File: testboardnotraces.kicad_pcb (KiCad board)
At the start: 2 copper layers, 88 x 96 mm, 75 parts, among them J1 Conn_02x05_Odd_Even, J2 Conn_01x06, J3 Thruster_Connection, Q1 SCT2450KEC, SW1 PTS645SM43SMTR92_LFS, U1 PIC18F47K40, U10 INA233, U11 INA233, U12 TPS2557, U13 EMCO-Q50-5, U14 TPS2557, U15 EMCO-Q50-5, U16 MAX6675, U2 MAX6816, U3 WPMDM171050601, U4 WPMDM171050601, U5 MAX5483, U6 EMCO-Q10-5, U7 INA233, U8 INA233, U9 INA233

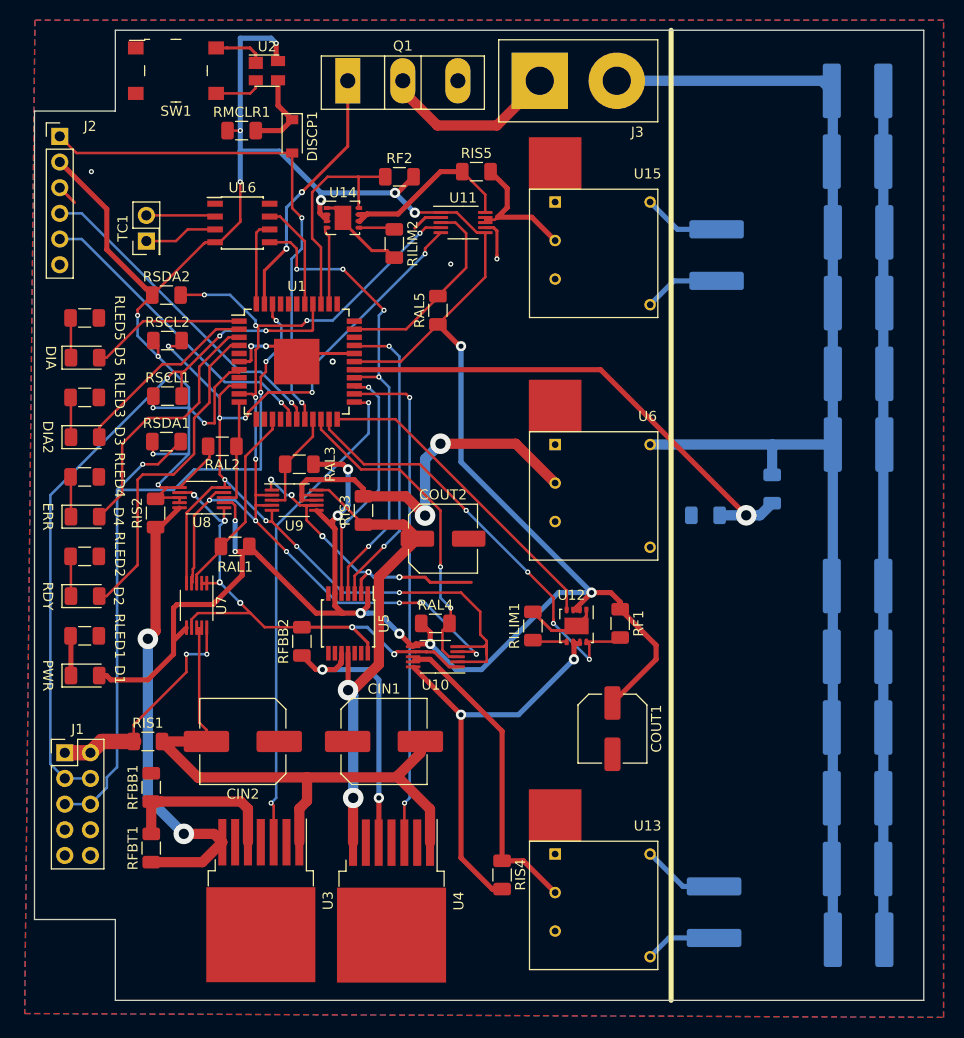
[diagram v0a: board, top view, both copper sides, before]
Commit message: Board design 1
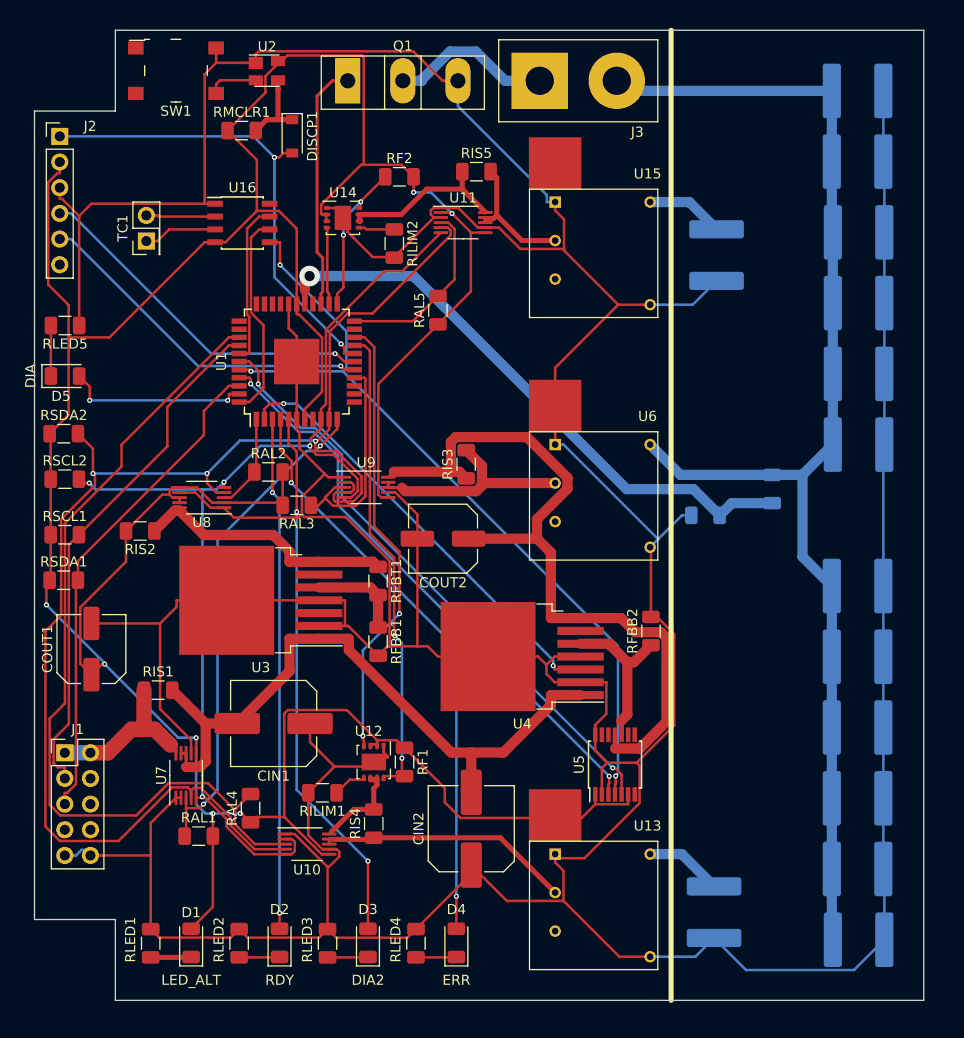
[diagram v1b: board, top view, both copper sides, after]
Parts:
- D1: value PWR -> LED_ALT
- moved RLED3 59.1 mm to (127.0, 139.3), turned to 270 degrees
- moved D3 57.3 mm to (131.0, 139.3), turned to 90 degrees
- moved RLED4 56.6 mm to (135.8, 139.3), turned to 270 degrees
- moved D4 55.9 mm to (139.8, 139.3), turned to 90 degrees
- moved COUT1 52.2 mm to (103.6, 110.2), turned to 90 degrees
- moved RLED2 41.2 mm to (118.2, 139.3), turned to 270 degrees
- moved D2 39.3 mm to (122.2, 139.3), turned to 90 degrees
- moved RFBT1 34.7 mm to (132.0, 103.5), turned to 270 degrees
- moved RFBB2 34.6 mm to (159.0, 108.5)
- moved RLED1 31.1 mm to (109.5, 139.3), turned to 270 degrees
- moved U5 29.9 mm to (155.4, 121.7), turned to 90 degrees
- moved U3 29.7 mm to (120.4, 105.4), turned to 180 degrees
- moved RAL1 28.9 mm to (114.2, 128.8)
- moved D1 28.5 mm to (113.5, 139.3), turned to 90 degrees
- moved U4 27.4 mm to (146.3, 111.0), turned to 180 degrees
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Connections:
- D2 pad 2: RDY_LED -> /RDY_LED
- D3 pad 2: DIA2_LED -> /DIA2_LED
- D4 pad 2: ERR_LED -> /ERR_LED
- D5 pad 2: DIA_LED -> /DIA_LED
- J1 pad 4: SCL1 -> (no net)
- J1 pad 6: SDA1 -> (no net)
- U1 pad 1: DIA_LED -> U8_ALERT
- U1 pad 11: U8_ALERT -> U7_ALERT
- U1 pad 14: U7_ALERT -> (no net)
- U1 pad 15: (no net) -> U9_ALERT
- U1 pad 19: U9_ALERT -> U12_FAULT
- U1 pad 2: DIA2_LED -> U4_EN
- U1 pad 20: U10_ALERT -> U12_EN
- U1 pad 21: U12_FAULT -> (no net)
- U1 pad 22: U12_EN -> U11_ALERT
- U1 pad 23: U3_EN -> U14_FAULT
- U1 pad 24: U4_EN -> U14_EN
- U1 pad 25: U5_DIN -> THRUST_CONTROL
- U1 pad 26: SCLK -> (no net)
- U1 pad 3: ERR_LED -> /RDY_LED
- U1 pad 30: U5_CS -> (no net)
- U1 pad 32: U11_ALERT -> (no net)
- U1 pad 35: U14_EN -> (no net)
- U1 pad 36: U14_FAULT -> U10_ALERT
- U1 pad 39: (no net) -> U5_DIN
- U1 pad 4: RDY_LED -> /ERR_LED
- U1 pad 40: (no net) -> SCLK
- U1 pad 41: (no net) -> U5_CS
- U1 pad 43: THRUST_CONTROL -> /DIA_LED
- U1 pad 5: (no net) -> /DIA2_LED
- U3 pad 3: U3_EN -> (no net)
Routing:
- net GND: track 224.4 -> 623.6 mm, vias 17 -> 0
- net /ERR_LED: track 0.00 -> 57.7 mm, vias 0 -> 2
- net /DIA2_LED: track 0.00 -> 53.7 mm, vias 0 -> 2
- net U10_ALERT: track 32.5 -> 85.2 mm, vias 2 -> 0
- net /RDY_LED: track 0.00 -> 50.7 mm, vias 0 -> 2
- net U3_EN: track 49.0 -> 0.00 mm, vias 2 -> 0
- net SDA2: track 101.3 -> 143.0 mm, vias 12 -> 3
- net U5_DIN: track 23.8 -> 60.1 mm
- net RDY_LED: track 33.4 -> 0.00 mm
- net /U12_VOUT: track 42.1 -> 9.62 mm, vias 2 -> 0
- net SCLK: track 48.1 -> 80.3 mm, vias 5 -> 3
- net U7_ALERT: track 19.3 -> 49.8 mm, vias 0 -> 2
- net U5_CS: track 30.2 -> 57.9 mm
- net SDA1: track 75.6 -> 49.3 mm, vias 4 -> 0
- net ERR_LED: track 26.2 -> 0.00 mm
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- removed copper zone on B.Cu, net GND
- removed copper zone on F.Cu, net GND
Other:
- net class 10mil: clearance 0 -> 0.127
- net class 12mil: clearance 0 -> 0.127
- net class 20mil: clearance 0 -> 0.127
- net class 40mil: clearance 0 -> 0.127
- net class 60mil: clearance 0 -> 0.127
- net class Default: clearance 0 -> 0.127
- rule trace_clearance: 0 -> 0.127
